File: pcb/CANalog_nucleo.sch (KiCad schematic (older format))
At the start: 2 parts

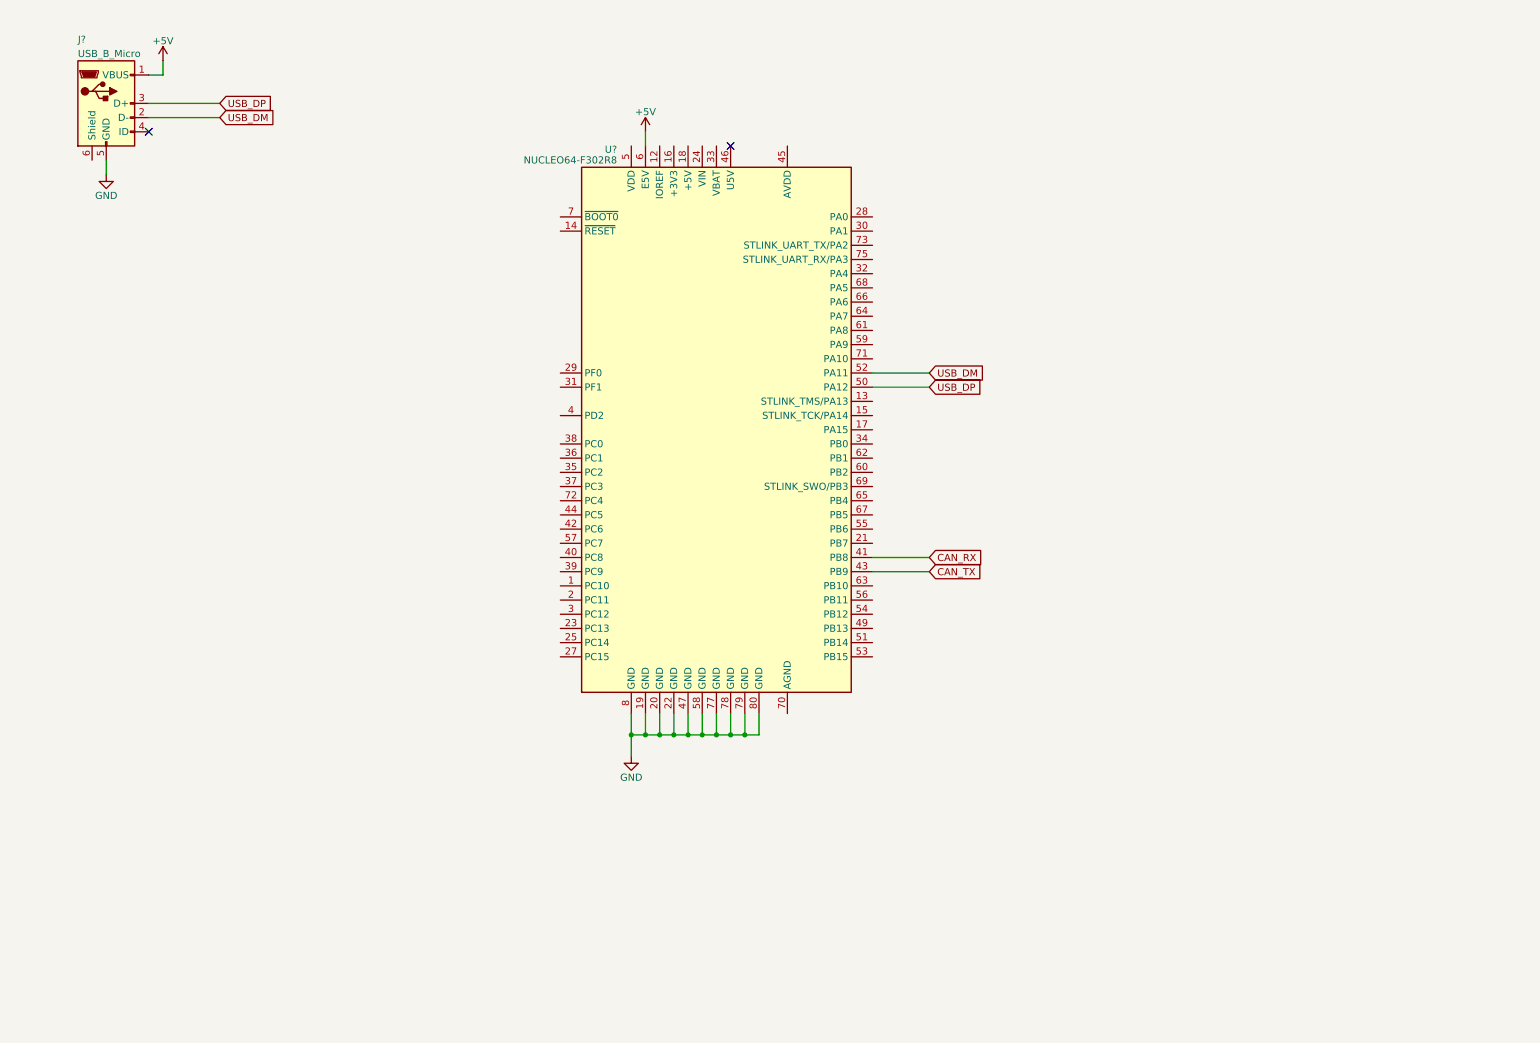
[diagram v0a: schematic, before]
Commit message: start schema
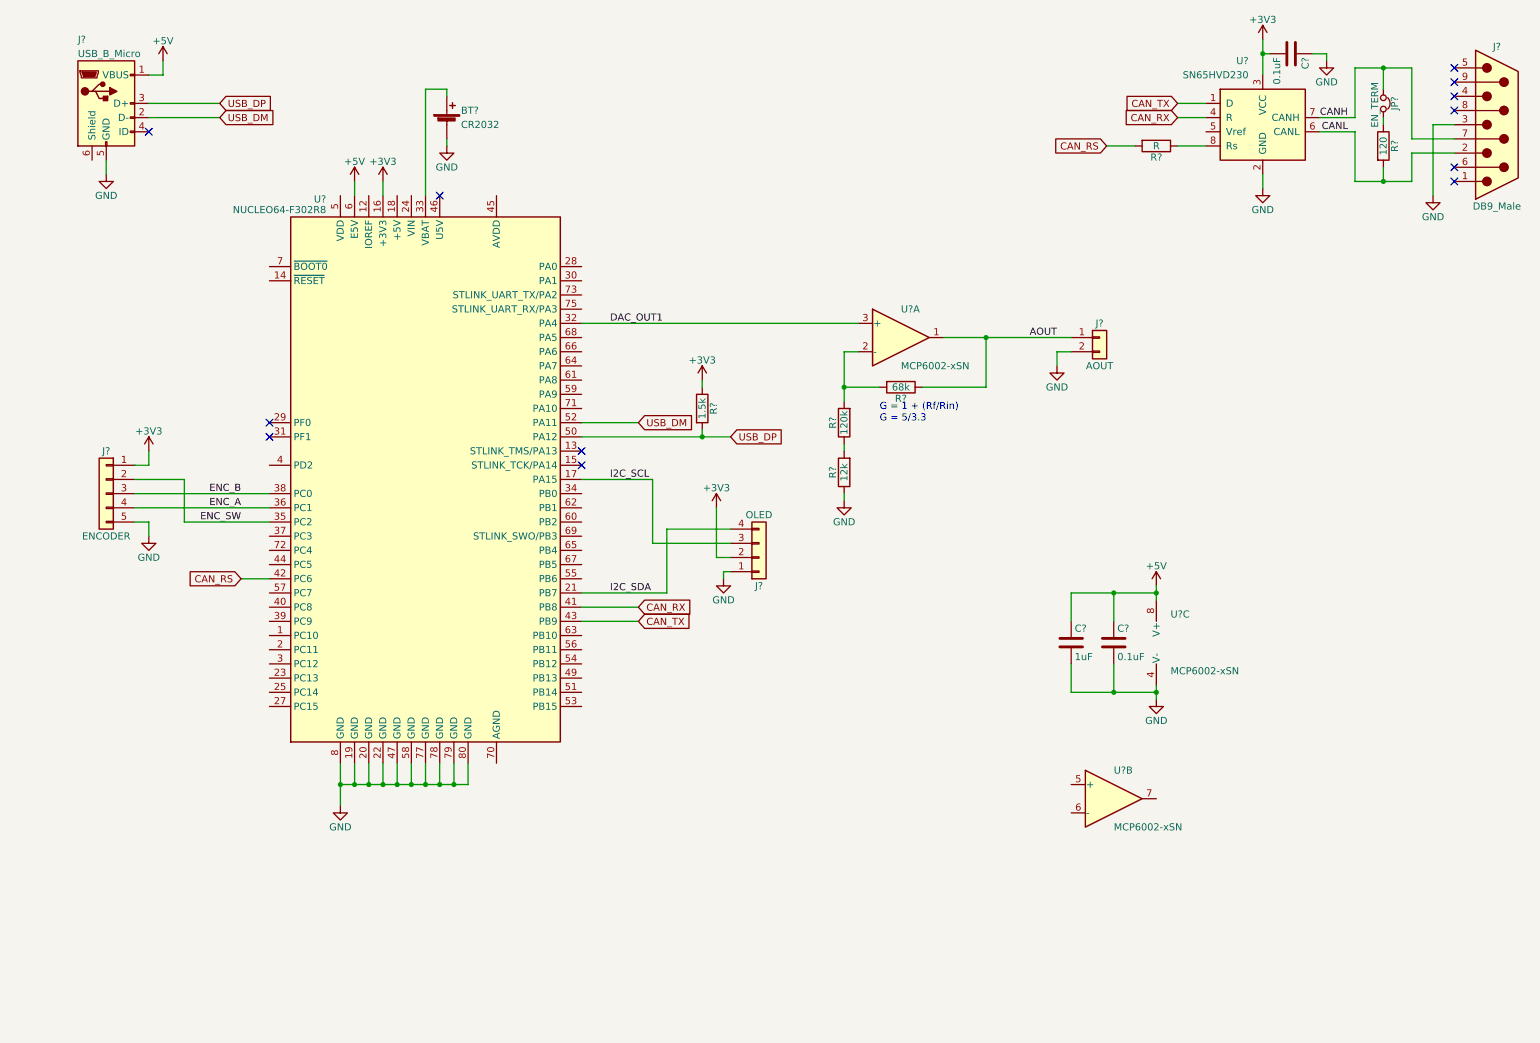
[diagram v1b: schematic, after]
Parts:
- added BT?: CR2032, symbol Device:Battery_Cell
- added C? (x2): 0.1uF, symbol Device:C
- added C?: 1uF, symbol Device:C
- added J?: DB9_Male, symbol Connector:DB9_Male
- added J?: ENCODER, symbol Connector_Generic:Conn_01x05
- added J?: OLED, symbol Connector_Generic:Conn_01x04
- added J?: AOUT, symbol Connector_Generic:Conn_01x02
- added JP?: EN_TERM, symbol Device:Jumper_NC_Small
- added R?: 1.5k, symbol Device:R
- added R?: R, symbol Device:R
- added R?: 120, symbol Device:R
- added R?: 68k, symbol Device:R
- added R?: 120k, symbol Device:R
- added R?: 12k, symbol Device:R
- added U?: SN65HVD230, Package_SO:SOIC-8_3.9x4.9mm_P1.27mm, symbol Interface_CAN_LIN:SN65HVD230
- added U? (x3): MCP6002-xSN, symbol Amplifier_Operational:MCP6002-xSN
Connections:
- net +5V: now also C?.1, C?.1, U?.8 (V+)
- net CAN_RX: now also U?.4 (R)
- net CAN_TX: now also U?.1 (D)
- net GND: now also BT?.2 (-), C?.1, C?.2, C?.2, J?.1 (Pin_1), J?.2 (Pin_2), J?.3, J?.5 (Pin_5), R?.1, U?.2 (GND), U?.4 (V-)
- net USB_DP: now also R?.2
- net +3V3: now reaches U?.16 (+3V3)
- net +3V3: now also C?.2, J?.1 (Pin_1), J?.2 (Pin_2), R?.1, U?.3 (VCC)
- net I2C_SCL: now reaches U?.17 (PA15)
- net I2C_SCL: now also J?.3 (Pin_3)
- net I2C_SDA: now reaches U?.21 (PB7)
- net I2C_SDA: now also J?.4 (Pin_4)
- net DAC_OUT1: now reaches U?.32 (PA4)
- net DAC_OUT1: now also U?.3 (+)
- net at U?.33 (VBAT): now also BT?.1 (+)
- net ENC_SW: now reaches U?.35 (PC2)
- net ENC_SW: now also J?.2 (Pin_2)
- net ENC_A: now reaches U?.36 (PC1)
- net ENC_A: now also J?.4 (Pin_4)
- net ENC_B: now reaches U?.38 (PC0)
- net ENC_B: now also J?.3 (Pin_3)
- net CAN_RS: now reaches U?.42 (PC6)
- net CAN_RS: now also R?.2
- new net: R?.1, U?.8 (Rs)
- new net: JP?.2, R?.1
- new net: R?.2, R?.2, U?.2 (-)
- new net: R?.1, R?.2
- new net AOUT: J?.1 (Pin_1), R?.1, U?.1
- new net CANH: J?.7, JP?.1, U?.7 (CANH)
- new net CANL: J?.2, R?.2, U?.6 (CANL)
- no-connect marks 2 -> 12
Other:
- note added: "G = 1 + (Rf/Rin)\nG = 5/3.3"
- moved on the sheet: U?

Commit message: schematic done
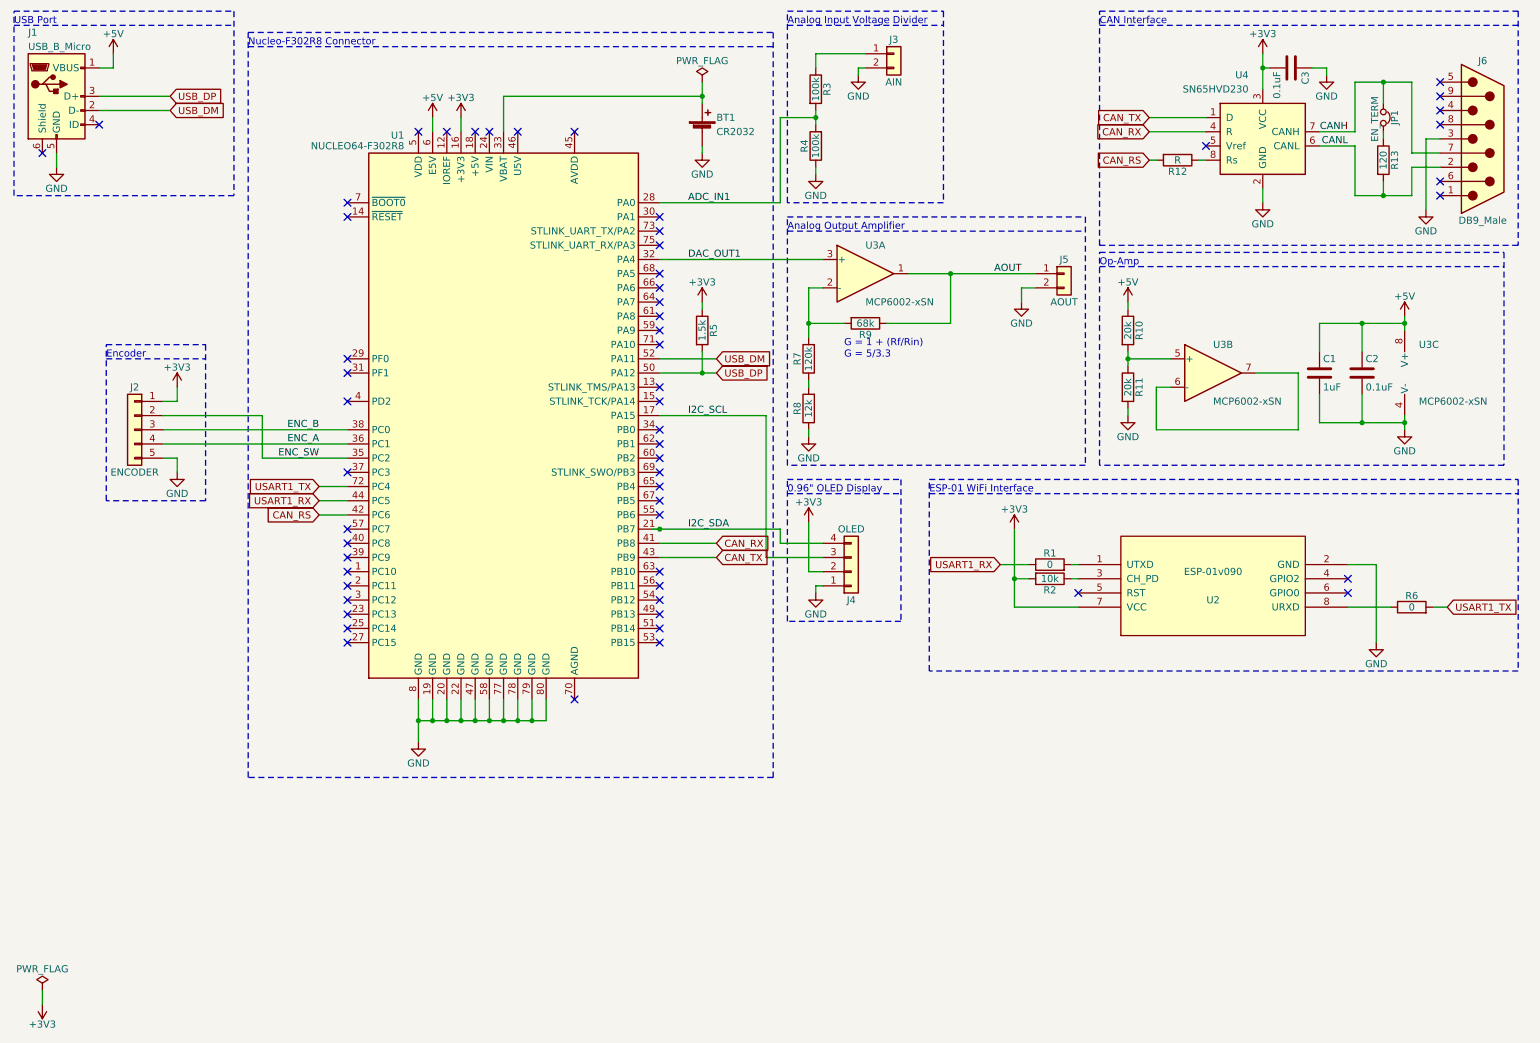
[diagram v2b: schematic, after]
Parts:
- added J3: AIN, pl_TerminalBlock:WJ127-5.0-2P, symbol Connector_Generic:Conn_01x02
- added R1, R6: 0, Resistor_SMD:R_0805_2012Metric_Pad1.20x1.40mm_HandSolder, symbol Device:R
- added R10, R11: 20k, Resistor_SMD:R_0805_2012Metric_Pad1.20x1.40mm_HandSolder, symbol Device:R
- added R2: 10k, Resistor_SMD:R_0805_2012Metric_Pad1.20x1.40mm_HandSolder, symbol Device:R
- added R3, R4: 100k, Resistor_SMD:R_0805_2012Metric_Pad1.20x1.40mm_HandSolder, symbol Device:R
- added U2: ESP-01v090, ESP8266:ESP-01, symbol ESP8266:ESP-01v090
- BT1: renamed from BT?; footprint (none) -> Battery:BatteryHolder_Keystone_103_1x20mm
- C1, C2, C3: renamed from C?; footprint (none) -> Capacitor_SMD:C_0805_2012Metric_Pad1.18x1.45mm_HandSolder
- J1: renamed from J?; footprint (none) -> Connector_USB:USB_Micro-B_Amphenol_10103594-0001LF_Horizontal
- J2: renamed from J?; footprint (none) -> Connector_PinHeader_2.54mm:PinHeader_1x05_P2.54mm_Vertical
- J4: renamed from J?; footprint (none) -> Connector_PinHeader_2.54mm:PinHeader_1x04_P2.54mm_Vertical
- J5: renamed from J?; footprint (none) -> pl_TerminalBlock:WJ127-5.0-2P
- J6: renamed from J?; footprint (none) -> Connector_Dsub:DSUB-9_Male_Horizontal_P2.77x2.84mm_EdgePinOffset7.70mm_Housed_MountingHolesOffset9.12mm
- JP1: renamed from JP?; footprint (none) -> Connector_PinHeader_2.54mm:PinHeader_1x02_P2.54mm_Vertical
- R12, R13, R5, R7, R8, R9: renamed from R?; footprint (none) -> Resistor_SMD:R_0805_2012Metric_Pad1.20x1.40mm_HandSolder
- U3: renamed from U?; footprint (none) -> Package_SO:SOIC-8_3.9x4.9mm_P1.27mm
- gave numbers to parts that had none: 2
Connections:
- net +3V3: now also R2.2, U2.7 (VCC)
- net +5V: now also R10.1
- net GND: now also J3.2 (Pin_2), R11.2, R4.1, U2.2 (GND)
- net ADC_IN1: now reaches U1.28 (PA0)
- net ADC_IN1: now also R3.2, R4.2
- net USART1_RX: now reaches U1.44 (PC5)
- net USART1_RX: now also R1.1
- net USART1_TX: now reaches U1.72 (PC4)
- net USART1_TX: now also R6.2
- net at U3.5 (+): now also R10.2, R11.1
- net at U3.6 (-): now also U3.7
- new net: R1.2, U2.1 (UTXD)
- new net: R2.1, U2.3 (CH_PD)
- new net: R6.1, U2.8 (URXD)
- new net: J3.1 (Pin_1), R3.1
- no-connect marks 12 -> 58
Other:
- note added: "0.96" OLED Display"
- note added: "Analog Input Voltage Divider"
- note added: "Analog Output Amplifier"
- note added: "CAN Interface"
- note added: "ESP-01 WiFi Interface"
- note added: "Encoder"
- note added: "Nucleo-F302R8 Connector"
- note added: "Op-Amp"
- note added: "USB Port"
- moved on the sheet: BT1, C1, C2, C3, J1, J2, J4, J5, J6, JP1, R12, R13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

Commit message: quickand dirty prototype
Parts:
- U1: footprint Module:ST_Morpho_Connector_144_STLink -> pl_Nucleo:nucleo-f302r8
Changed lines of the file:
@@
 F 0 "U1" H 3300 5375 50  0000 R CNN
 F 1 "NUCLEO64-F302R8" H 3300 5300 50  0000 R CNN
-F 2 "Module:ST_Morpho_Connector_144_STLink" H 4550 1500 50  0001 L CNN
+F 2 "pl_Nucleo:nucleo-f302r8" H 4550 1500 50  0001 L CNN
 F 3 "" H 3100 2000 50  0001 C CNN
 	1    4000 3400
@@
 	6200 850  6200 950
 $Comp
-L power:GND #PWR?
+L power:GND #PWR0102
 U 1 1 60809ED1
 P 6200 1700
-F 0 "#PWR?" H 6200 1450 50  0001 C CNN
+F 0 "#PWR0102" H 6200 1450 50  0001 C CNN
 F 1 "GND" H 6200 1550 50  0000 C CNN
 F 2 "" H 6200 1700 50  0001 C CNN
